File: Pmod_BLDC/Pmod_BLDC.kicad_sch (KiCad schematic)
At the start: 0 parts

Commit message: BLDC schematics
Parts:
- added C1, C2, C3, C4, C5, C6: C, Capacitor_SMD:C_0603_1608Metric_Pad1.08x0.95mm_HandSolder, symbol Device:C
- added D1, D2, D4: MMBD7000LT1G, SOT96P237X111-3N, symbol samacsys:MMBD7000LT1G
- added IC1, IC2, IC3: S-5725ECBL0-M3T1U, SOT95P275X130-3N, symbol samacsys:S-5725ECBL0-M3T1U
- added J1: Screw_Terminal_01x03, TerminalBlock:TerminalBlock_Xinya_XY308-2.54-3P_1x03_P2.54mm_Horizontal, symbol Connector:Screw_Terminal_01x03
- added J2: Conn_02x06_Top_Bottom, Connector_PinHeader_2.54mm:PinHeader_2x06_P2.54mm_Horizontal, symbol Connector_Generic:Conn_02x06_Top_Bottom
- added R1, R6, R9: 4.7k, Resistor_SMD:R_0603_1608Metric_Pad0.98x0.95mm_HandSolder, symbol Device:R
- added R2, R3, R4, R5, R7, R8: 1k, Resistor_SMD:R_0603_1608Metric_Pad0.98x0.95mm_HandSolder, symbol Device:R
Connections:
- new net: D1.3 (K/A), R4.2, R5.1
- new net: IC2.3 (VOUT), R5.2, R6.2
- new net: D2.3 (K/A), R7.2, R8.1
- new net: IC3.3 (VOUT), R8.2, R9.2
- new net: IC1.3 (VOUT), R1.2, R2.2
- new net: C6.1, J2.3 (Pin_9), R7.1
- new net: C4.1, J2.1 (Pin_7), R3.1
- new net: D4.3 (K/A), R2.1, R3.2
- new net: C5.1, J2.2 (Pin_8), R4.1
- new net +3.3V: C1.1, C2.1, C3.1, D1.2 (K), D2.2 (K), D4.2 (K), IC1.2 (VDD), IC2.2 (VDD), IC3.2 (VDD), R1.1, R6.1, R9.1
- new net GND: C1.2, C2.2, C3.2, C4.2, C5.2, C6.2, D1.1 (A), D2.1 (A), D4.1 (A), IC1.1 (VSS), IC2.1 (VSS), IC3.1 (VSS)

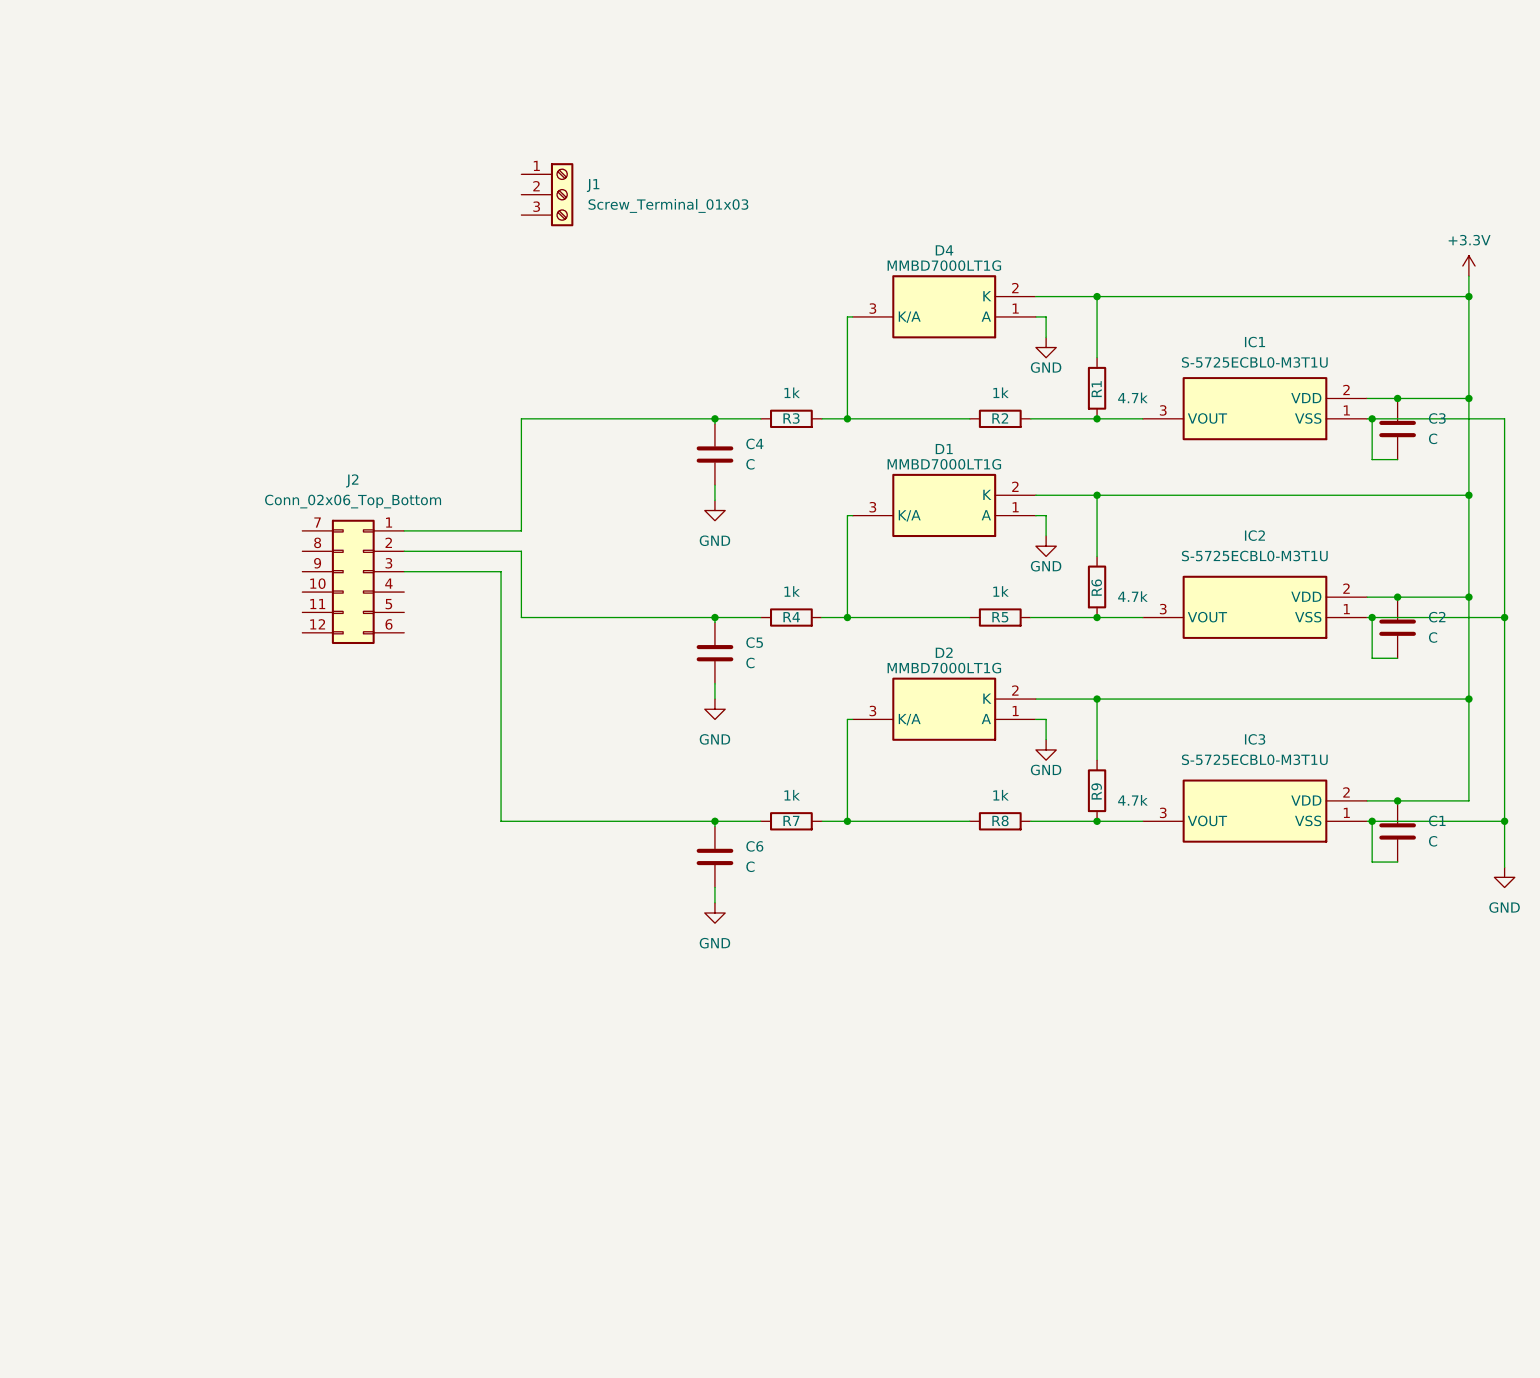
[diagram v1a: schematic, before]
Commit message: 0615
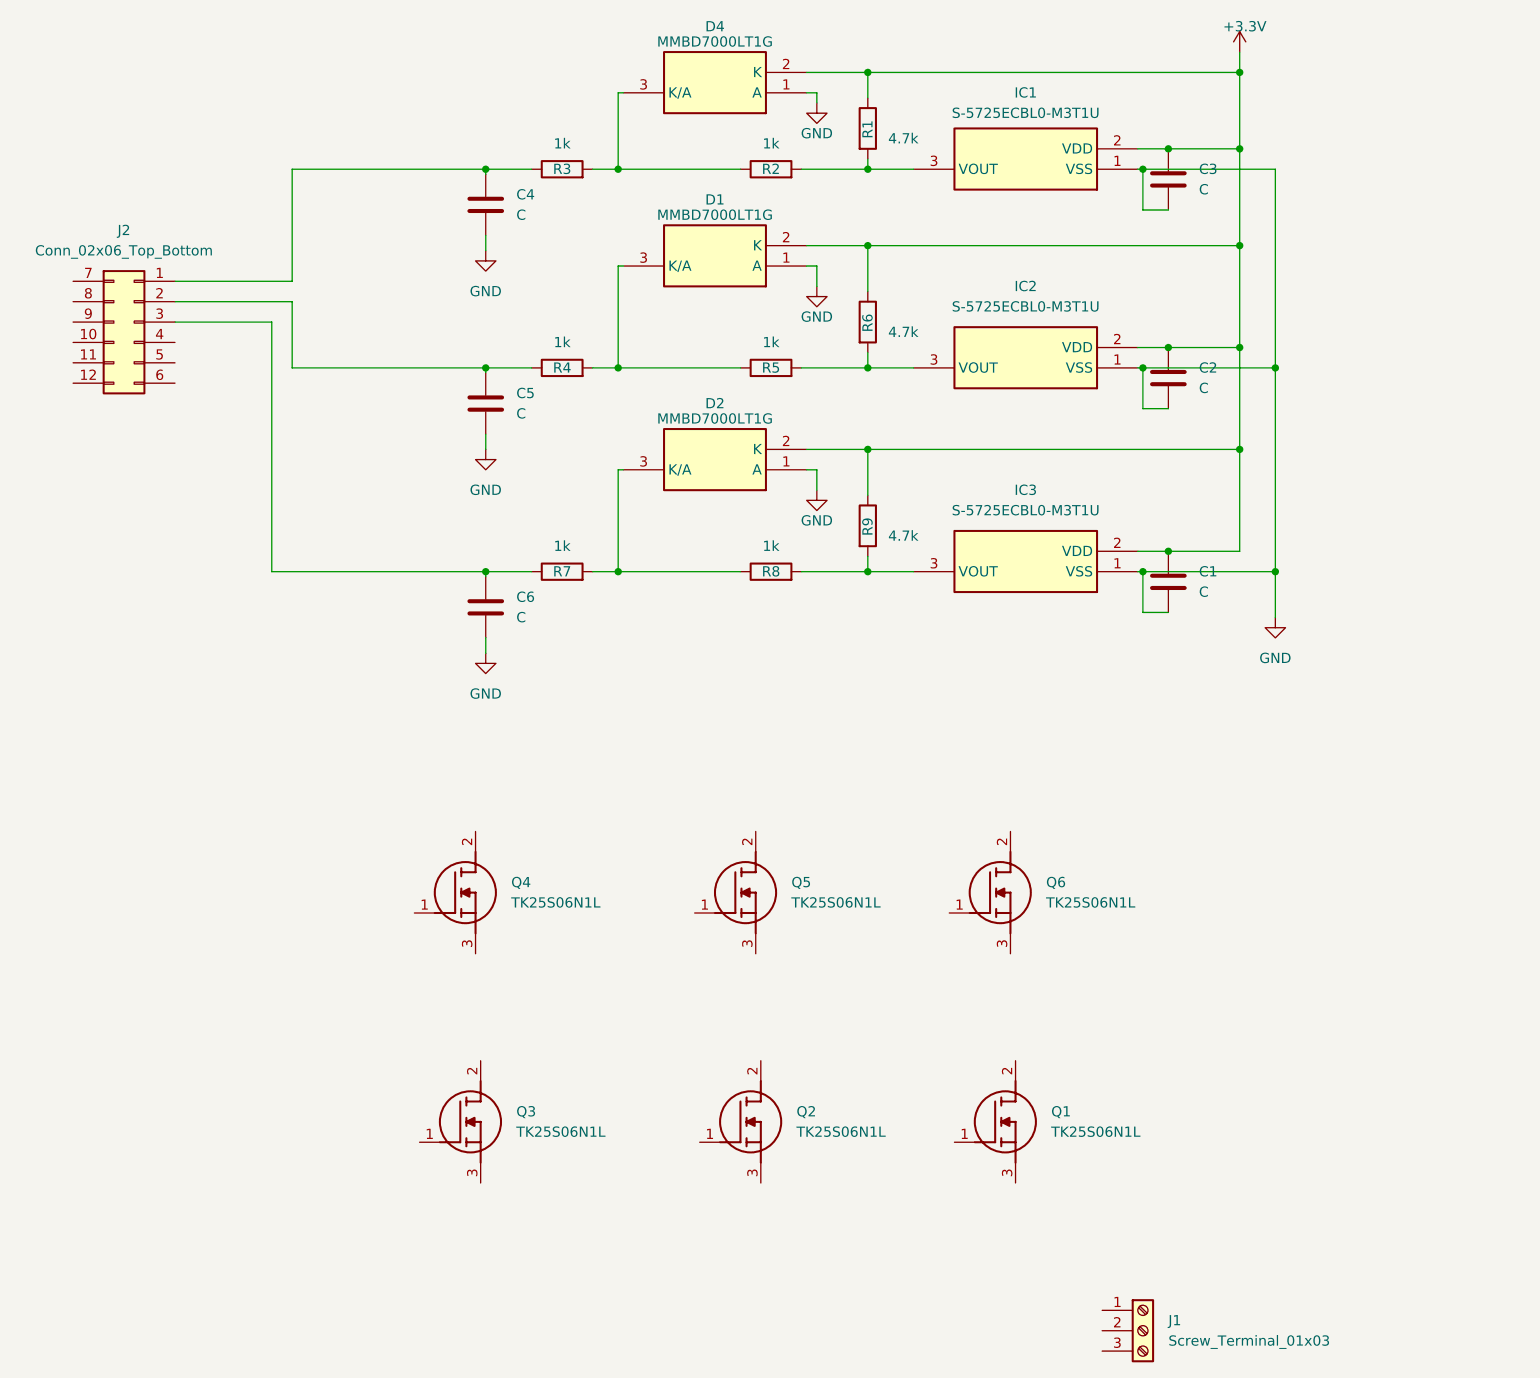
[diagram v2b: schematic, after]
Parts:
- added Q1, Q2, Q3, Q4, Q5, Q6: TK25S06N1L, TK7S10N1ZLXHQ, symbol samacsys:TK25S06N1L
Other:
- moved on the sheet: C1, C2, C3, C4, C5, C6, D1, D2, D4, IC1, IC2, IC3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

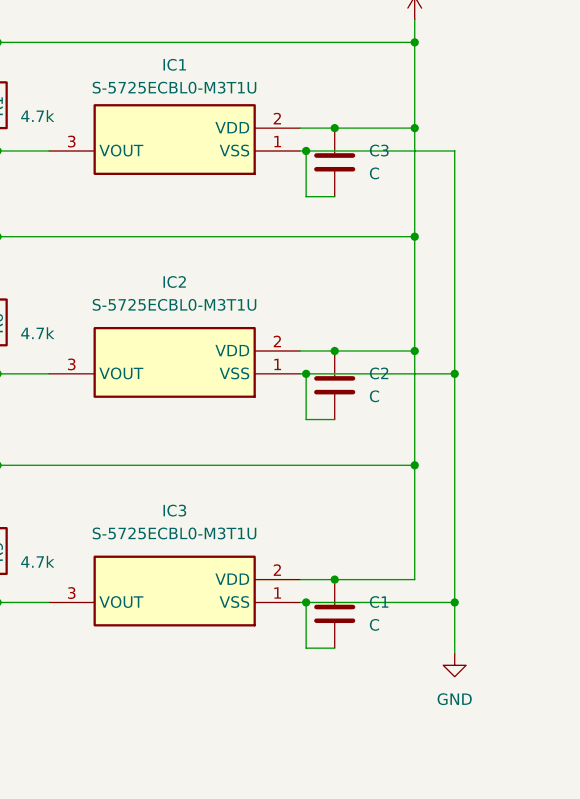
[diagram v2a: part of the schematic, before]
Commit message: 0617
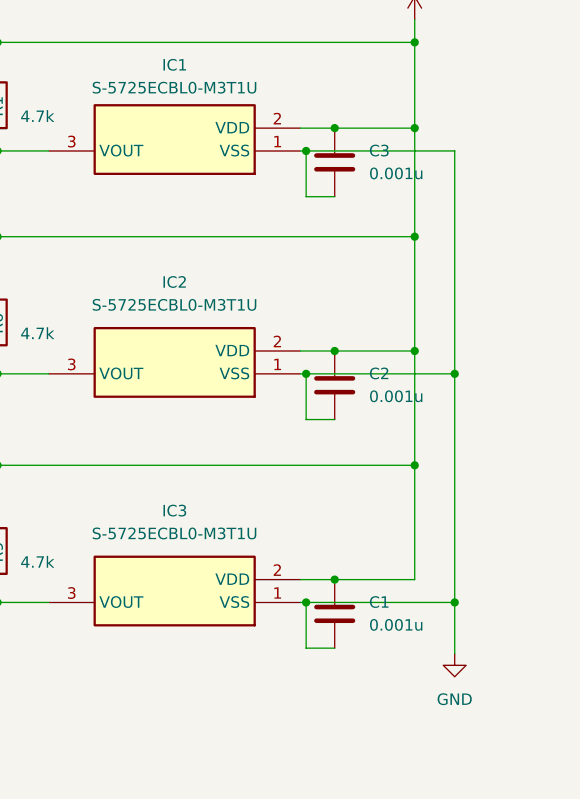
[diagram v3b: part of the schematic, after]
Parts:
- C1, C2, C3: value C -> 0.001u
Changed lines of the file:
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@@
 			)
 		)
-		(property "Value" "C"
+		(property "Value" "0.001u"
 			(at 161.925 36.1949 0)
 			(effects
@@
 			)
 		)
-		(property "Value" "C"
+		(property "Value" "0.001u"
 			(at 161.925 86.3599 0)
 			(effects
@@
 			)
 		)
-		(property "Value" "C"
+		(property "Value" "0.001u"
 			(at 161.925 60.9599 0)
 			(effects
